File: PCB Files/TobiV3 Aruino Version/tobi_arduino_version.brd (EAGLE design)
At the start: 103 x 74 mm, 45 parts

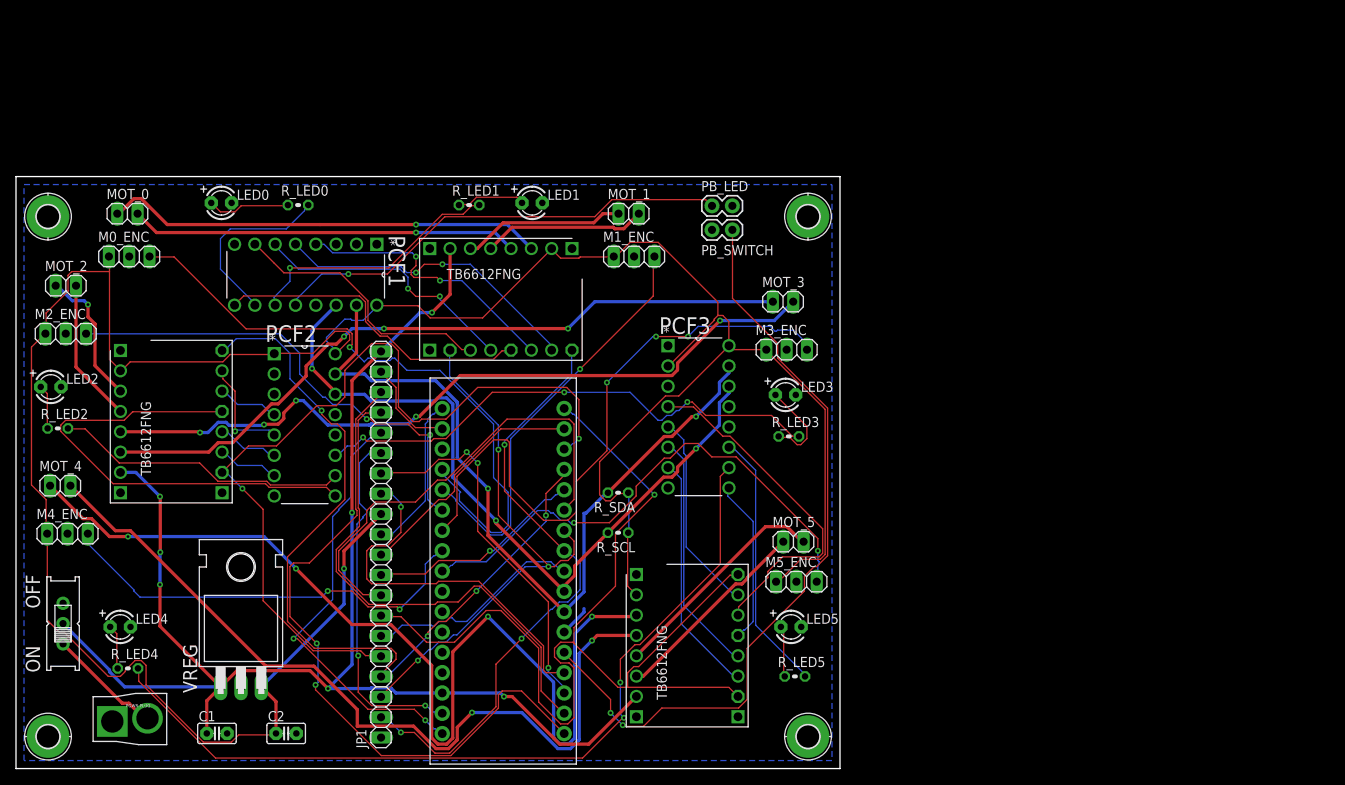
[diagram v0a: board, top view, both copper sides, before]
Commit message: let's try this again
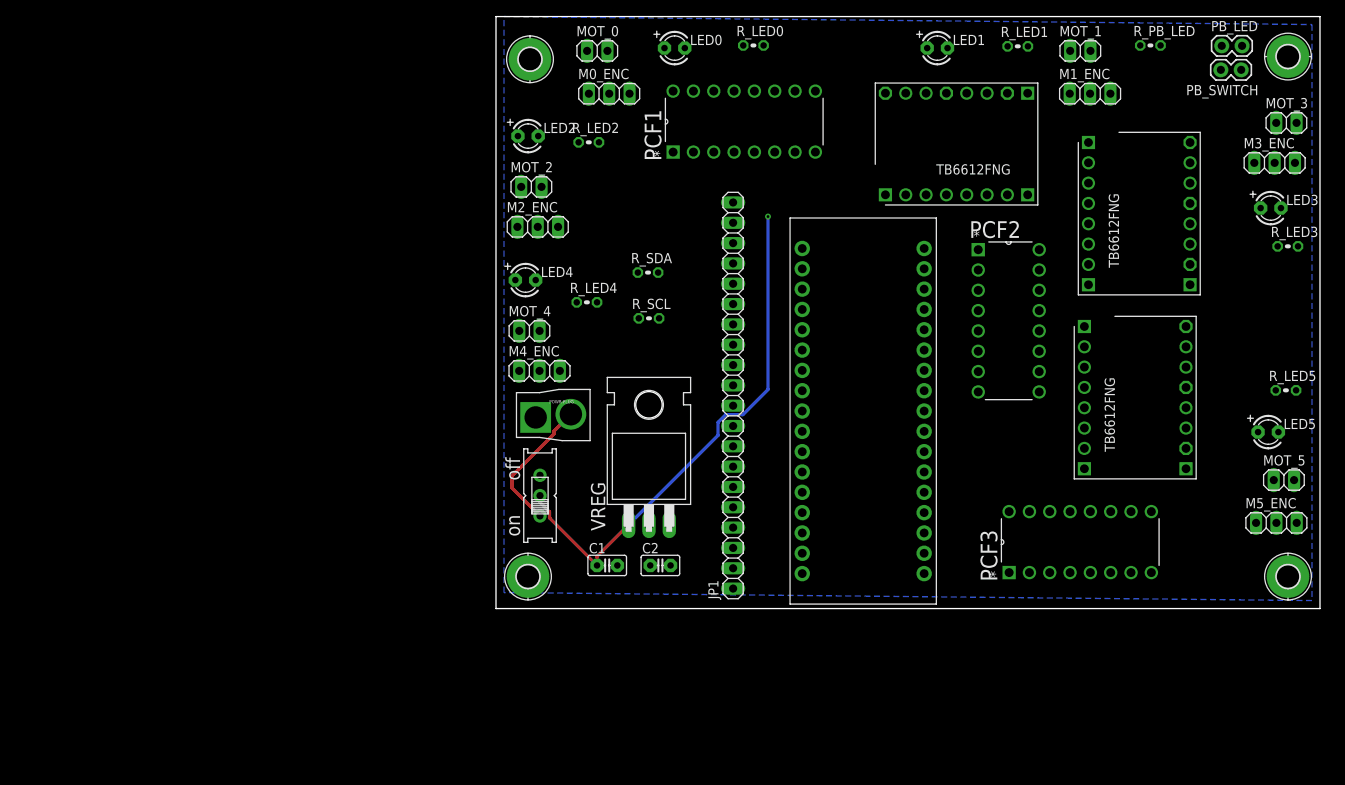
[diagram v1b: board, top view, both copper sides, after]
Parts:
- added R_PB_LED: 1000, resistor:0204V
- R_LED0, R_LED1, R_LED2, R_LED3, R_LED4, R_LED5: value (none) -> 1000
- R_SCL, R_SDA: value (none) -> 100000
- moved H3 176.8 mm to (156.0, 95.0), turned to 270 degrees
- moved DRIVER2 123.8 mm to (129.8, 65.2)
- moved H4 91.5 mm to (61.2, 94.7), turned to 0 degrees
- moved PCF2 89.0 mm to (124.9, 53.1)
- moved DRIVER1 77.4 mm to (124.7, 76.5), turned to 90 degrees
- moved PCF1 77.4 mm to (96.9, 90.7), turned to 90 degrees
- moved R_LED2 75.4 mm to (68.6, 84.3)
- moved H1 75.0 mm to (61.0, 30.0), turned to 0 degrees
- moved H2 75.0 mm to (156.0, 30.0)
- moved R_LED4 73.4 mm to (68.4, 64.3)
- moved R_LED1 71.4 mm to (122.2, 96.3)
- moved R_LED5 71.0 mm to (155.7, 53.3)
- moved LED2 67.4 mm to (61.0, 85.1)
- moved PB_LED 66.8 mm to (147.7, 96.3)
- moved MOT_3 66.8 mm to (155.8, 86.7)
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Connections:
- removed net N$2: LED1.A, R_LED1.1
- removed net N$3: LED2.A, R_LED2.1
- removed net N$4: LED3.A, R_LED3.1
- removed net N$5: LED4.A, R_LED4.1
- removed net N$6: LED5.A, R_LED5.1
- net GND: no longer LED0.K, LED1.K, LED2.K, LED3.K, LED4.K, LED5.K, PB_LED.2
- net LED0: now also LED0.K, R_LED0.1
- net LED1: now also LED1.K, R_LED1.1
- net LED2: now also LED2.K, R_LED2.1
- net LED3: now also LED3.K, R_LED3.1
- net LED4: now also LED4.K, R_LED4.1
- net LED5: now also LED5.K, R_LED5.1
- net N$1: now also PB_LED.2, R_PB_LED.2; no longer LED0.A, R_LED0.1
- net PB_LED: now also R_PB_LED.1; no longer PB_LED.1
- net SCL: now also R_SCL.1; no longer R_SCL.2
- net SDA: now also R_SDA.1; no longer R_SDA.2
- net VCC: now also LED0.A, LED1.A, LED2.A, LED3.A, LED4.A, LED5.A, PB_LED.1, R_SCL.2, R_SDA.2; no longer R_SCL.1, R_SDA.1
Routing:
- net VCC: track 335.5 -> 0.00 mm, vias 1 -> 0
- net M5_PWM: track 132.9 -> 0.00 mm, vias 1 -> 0
- net M4_A: track 129.9 -> 0.00 mm, vias 4 -> 0
- net V_MOT: track 184.1 -> 65.4 mm, vias 7 -> 1
- net M3_PWM: track 107.2 -> 0.00 mm, vias 2 -> 0
- net LED4: track 105.8 -> 0.00 mm, vias 2 -> 0
- net M2_PWM: track 104.9 -> 0.00 mm, vias 4 -> 0
- net M4_B: track 102.4 -> 0.00 mm, vias 2 -> 0
- net SDA: track 98.5 -> 0.00 mm, vias 2 -> 0
- net RESET: track 97.1 -> 0.00 mm, vias 2 -> 0
- net M3_B: track 94.7 -> 0.00 mm, vias 5 -> 0
- net SCL: track 93.1 -> 0.00 mm, vias 3 -> 0
- net M3_A: track 90.1 -> 0.00 mm, vias 3 -> 0
- net MOSI: track 85.9 -> 0.00 mm, vias 2 -> 0
- net M0_ENC: track 80.2 -> 0.00 mm, vias 1 -> 0
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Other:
- board text added: "off"
- board text added: "on"
- board text removed: "OFF"
- board text removed: "ON"
- board text removed: "TOBI v4 Tom Dodson"
- board text removed: "www.grasp.upenn.edu"
